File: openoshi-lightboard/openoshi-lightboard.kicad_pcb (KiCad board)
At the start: 2 copper layers, 30 x 30 mm, 26 parts, among them J1 USB_C_Receptacle_PowerOnly_6P, Q1 CSD17484F4, Q2 CSD17484F4, Q3 CSD17484F4, Q4 CSD17484F4, SW1 SW_Push, SW2 SW_Push, U1 CH32V003FxUx, U2 TLV61070ADBV, U3 MCP73831-2-OT

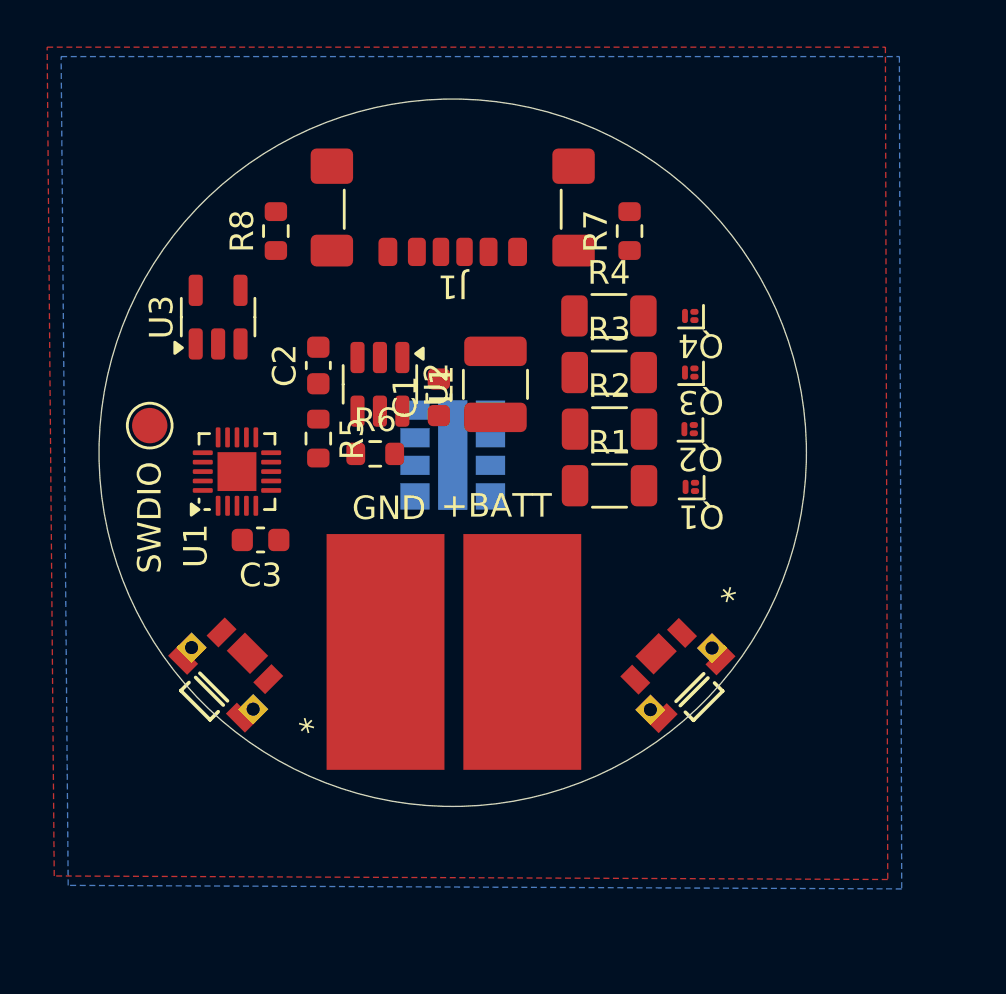
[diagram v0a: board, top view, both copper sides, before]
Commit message: Safety upgrades all around
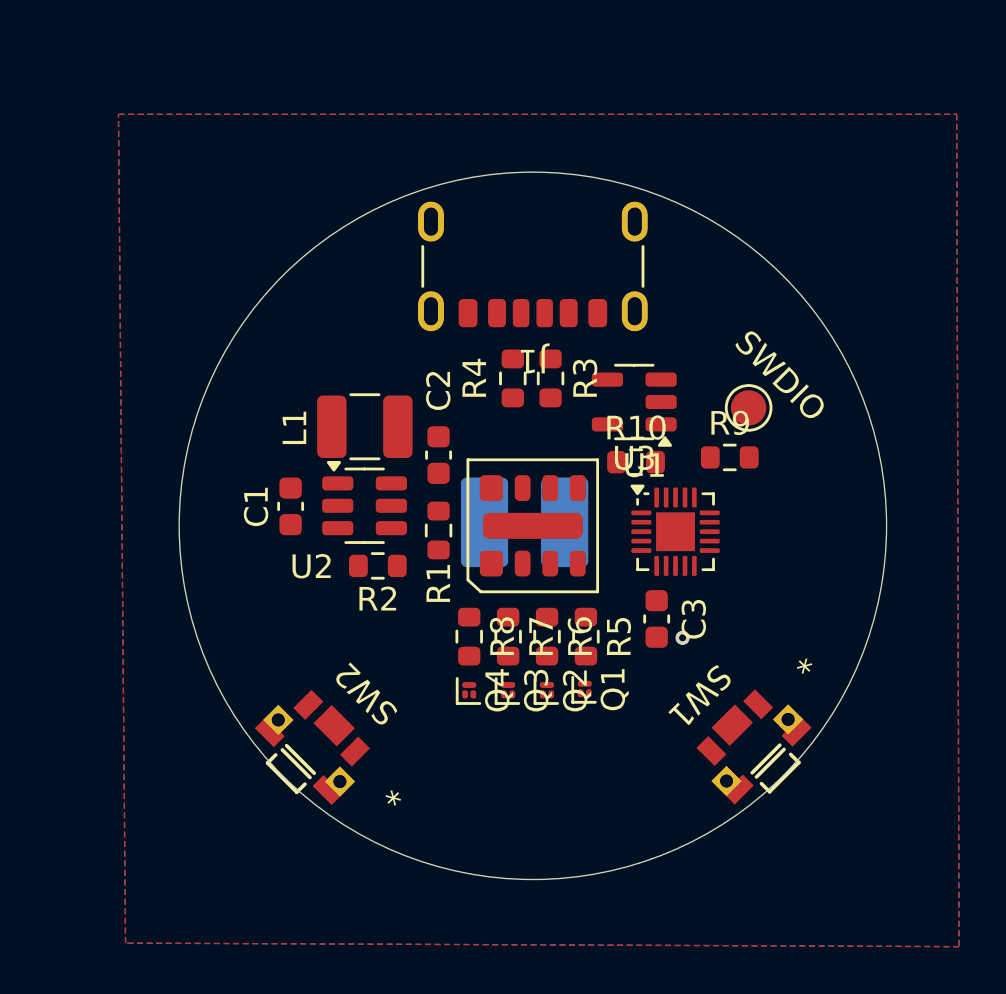
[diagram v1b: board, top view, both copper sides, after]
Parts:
- removed LED1: L1MC-RGB5080500MP0, openoshi-lightboard:5050RGBW_LUL
- added D1: Lumileds_5052RGBW, openoshi-lightboard:LED_Lumileds_5052RGBW_LGA9_5.0x5.2mm_P0.5mm, F.Cu at (150.4, 98.4)
- added R10: 2k, Resistor_SMD:R_0603_1608Metric, F.Cu at (154.4, 97.3)
- added R9: 220, Resistor_SMD:R_0603_1608Metric, F.Cu at (158.3, 97.1)
- J1: footprint Connector_USB:USB_C_Receptacle_GCT_USB4135-GF-A_6P_TopMnt_Horizontal -> Connector_USB:USB_C_Receptacle_GCT_USB4125-xx-x_6P_TopMnt_Horizontal
- L1: value 4.7uH -> L
- Q1, Q2, Q3, Q4: value CSD17484F4 -> PMZ600UNEYL
- R5: renamed from R1; value R -> 118; footprint Resistor_SMD:R_1206_3216Metric -> Resistor_SMD:R_0603_1608Metric
- R6: renamed from R2; value R -> 69.8; footprint Resistor_SMD:R_1206_3216Metric -> Resistor_SMD:R_0603_1608Metric
- R7: renamed from R3; value R -> 69.8; footprint Resistor_SMD:R_1206_3216Metric -> Resistor_SMD:R_0603_1608Metric
- R8: renamed from R4; value R -> 69.8; footprint Resistor_SMD:R_1206_3216Metric -> Resistor_SMD:R_0603_1608Metric
- TP2, TP3: footprint Connector_Wire:SolderWirePad_1x01_SMD_5x10mm -> TestPoint:TestPoint_Keystone_5019_Miniature; moved to B.Cu
- U2: value TLV61070ADBV -> TLV61220
- moved TP1 25.4 mm to (159.2, 95.0), turned to 135 degrees
- moved U1 18.8 mm to (156.1, 100.2), turned to 0 degrees
- moved Q4 18.4 mm to (147.3, 107.0), turned to 90 degrees
- moved U3 18.0 mm to (154.3, 94.8), turned to 180 degrees
- moved C3 17.1 mm to (155.2, 104.0), turned to 90 degrees
- moved Q3 15.5 mm to (148.9, 107.0), turned to 90 degrees
- moved R8 14.8 mm to (147.3, 104.7), turned to -90 degrees
- moved Q2 12.6 mm to (150.6, 107.0), turned to 90 degrees
- moved R7 12.0 mm to (148.9, 104.7), turned to -90 degrees
- moved R4 11.8 mm to (149.2, 93.8)
- moved Q1 9.68 mm to (152.2, 106.9), turned to 90 degrees
- moved TP3 9.38 mm to (151.3, 99.8), turned to 90 degrees
- moved R6 9.19 mm to (150.6, 104.7), turned to -90 degrees
- moved C1 7.81 mm to (139.7, 99.2)
- moved R3 7.09 mm to (150.8, 93.8)
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- renumbered R5 to R1, R6 to R2, R7 to R3, R8 to R4
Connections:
- net /VREG_FB renamed Net-(U2-V_{FB})
- SW1 pad 1: unconnected-(SW1-Pad1) -> /SW1_DET
- SW1 pad 2: unconnected-(SW1-Pad2) -> GND
- SW2 pad 1: unconnected-(SW2-Pad1) -> /SW2_DET
- SW2 pad 2: unconnected-(SW2-Pad2) -> GND
- U1 pad 15: /SWDIO -> Net-(U1-PD1)
- U3 pad 1: unconnected-(U3-STAT-Pad1) -> /CHG_STAT
- U3 pad 5: unconnected-(U3-PROG-Pad5) -> Net-(U3-PROG)
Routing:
- net GND: vias 0 -> 1
